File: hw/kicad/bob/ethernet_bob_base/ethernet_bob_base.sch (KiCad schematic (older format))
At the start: 14 parts, among them J1 DB9_Male, J2 Conn_01x02_Male, J3 Conn_01x02_Male, J4 Conn_01x02_Male, J5 Conn_01x04_Male, J6 Conn_01x04_Male, J7 Conn_01x04_Male, J8 Conn_01x04_Male, U2 TJA1021T, U3 MCP2551-I-SN, U4 MC33879A, U5 MC33879A

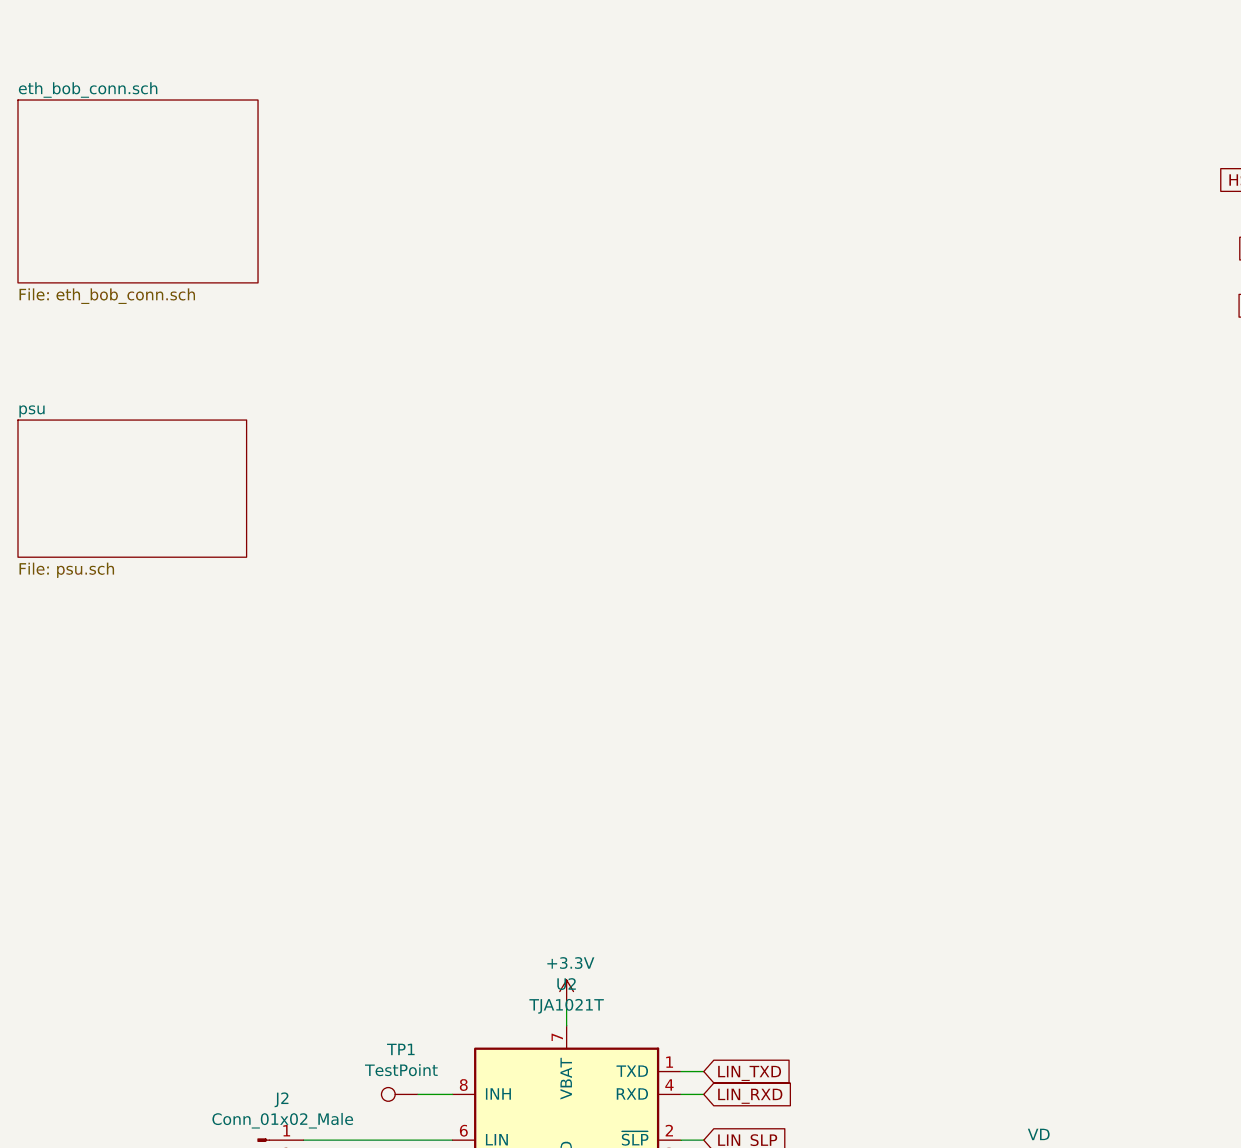
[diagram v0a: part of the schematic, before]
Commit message: routing...
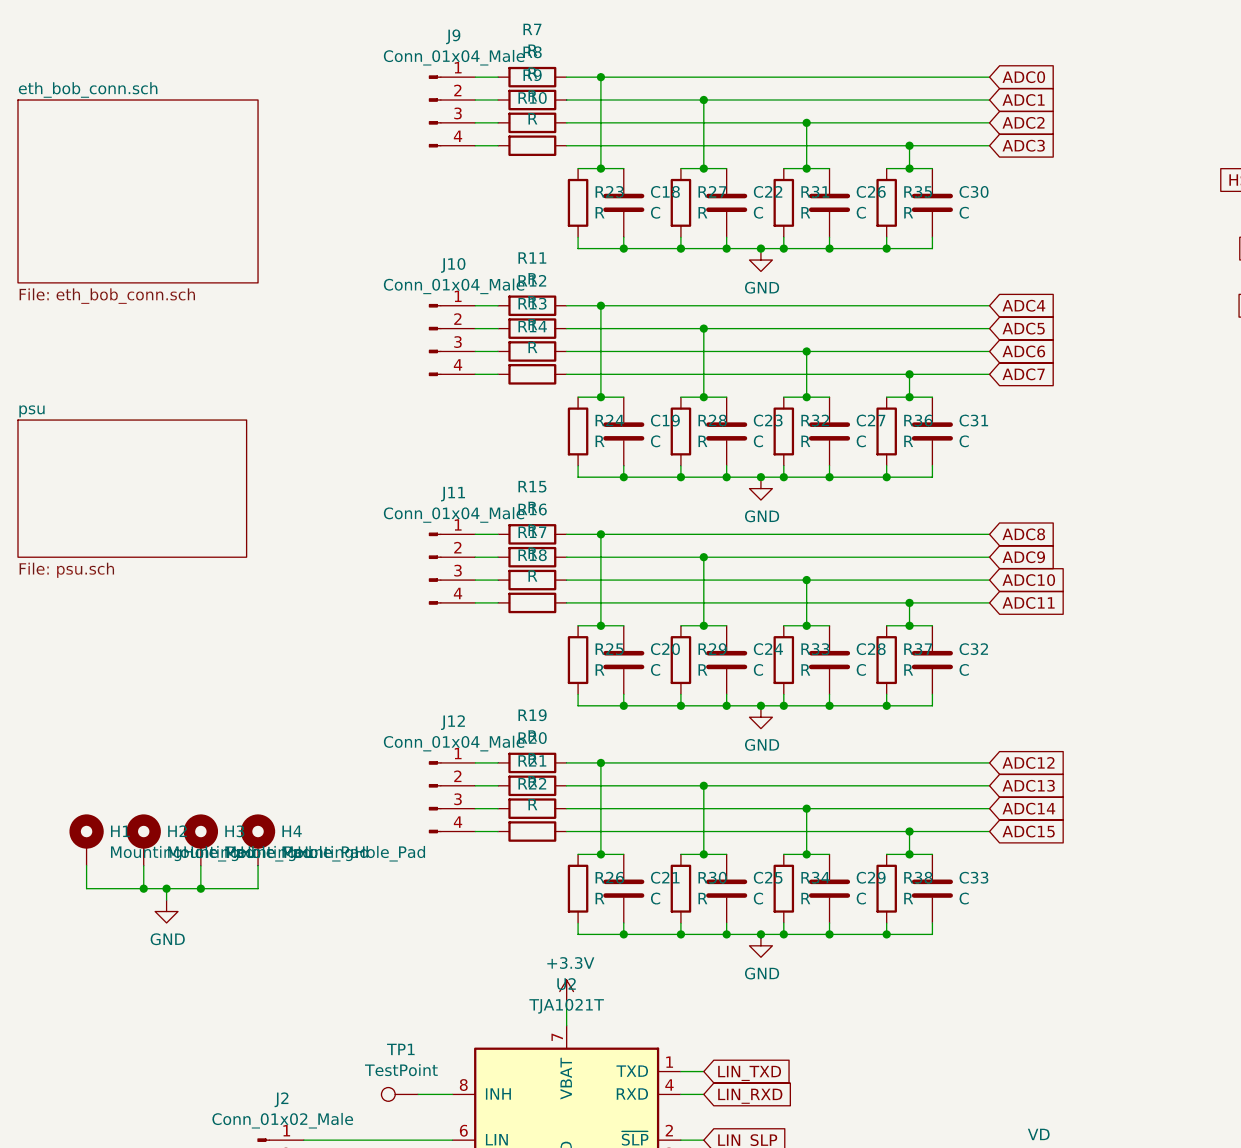
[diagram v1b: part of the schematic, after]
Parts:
- added C18, C19, C20, C21, C22, C23, C24, C25, C26, C27, C28, C29, C30, C31, C32, C33: C, stmbl-kicad-lib:C_0805, symbol stmbl:C
- added H1, H2, H3, H4: MountingHole_Pad, Mounting_Holes:MountingHole_3.2mm_M3_Pad_Via, symbol Mechanical:MountingHole_Pad
- added J10, J11, J12, J9: Conn_01x04_Male, stmbl-kicad-lib:RM3.5_1x4_UP, symbol Connector:Conn_01x04_Male
- added R10, R11, R12, R13, R14, R15, R16, R17, R18, R19, R20, R21, R22, R23, R24, R25, R26, R27, R28, R29, R30, R31, R32, R33, R34, R35, R36, R37, R38, R7, R8, R9: R, stmbl-kicad-lib:R_0603, symbol stmbl:R
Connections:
- net GND: now also C18.2, C19.2, C20.2, C21.2, C22.2, C23.2, C24.2, C25.2, C26.2, C27.2, C28.2, C29.2, C30.2, C31.2, C32.2, C33.2, H1.1, H2.1, H3.1, H4.1, R23.2, R24.2, R25.2, R26.2, R27.2, R28.2, R29.2, R30.2, R31.2, R32.2, R33.2, R34.2, R35.2, R36.2, R37.2, R38.2
- new net: J9.1 (Pin_1), R7.2
- new net: J9.2 (Pin_2), R8.2
- new net: J9.3 (Pin_3), R9.2
- new net: J9.4 (Pin_4), R10.2
- new net: J10.1 (Pin_1), R11.2
- new net: J10.2 (Pin_2), R12.2
- new net: J10.3 (Pin_3), R13.2
- new net: J10.4 (Pin_4), R14.2
- new net: J11.1 (Pin_1), R15.2
- new net: J11.2 (Pin_2), R16.2
- new net: J11.3 (Pin_3), R17.2
- new net: J11.4 (Pin_4), R18.2
- new net: J12.1 (Pin_1), R19.2
- new net: J12.2 (Pin_2), R20.2
- new net: J12.3 (Pin_3), R21.2
- new net: J12.4 (Pin_4), R22.2
- new net ADC0: C18.1, R23.1, R7.1
- new net ADC1: C22.1, R27.1, R8.1
- new net ADC10: C28.1, R17.1, R33.1
- new net ADC11: C32.1, R18.1, R37.1
- new net ADC12: C21.1, R19.1, R26.1
- new net ADC13: C25.1, R20.1, R30.1
- new net ADC14: C29.1, R21.1, R34.1
- new net ADC15: C33.1, R22.1, R38.1
- new net ADC2: C26.1, R31.1, R9.1
- new net ADC3: C30.1, R10.1, R35.1
- new net ADC4: C19.1, R11.1, R24.1
- new net ADC5: C23.1, R12.1, R28.1
- new net ADC6: C27.1, R13.1, R32.1
- new net ADC7: C31.1, R14.1, R36.1
- new net ADC8: C20.1, R15.1, R25.1
- new net ADC9: C24.1, R16.1, R29.1
